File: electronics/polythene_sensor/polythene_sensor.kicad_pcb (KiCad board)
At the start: 2 copper layers, 8 parts, among them J1 Conn_02x16_Counter_Clockwise

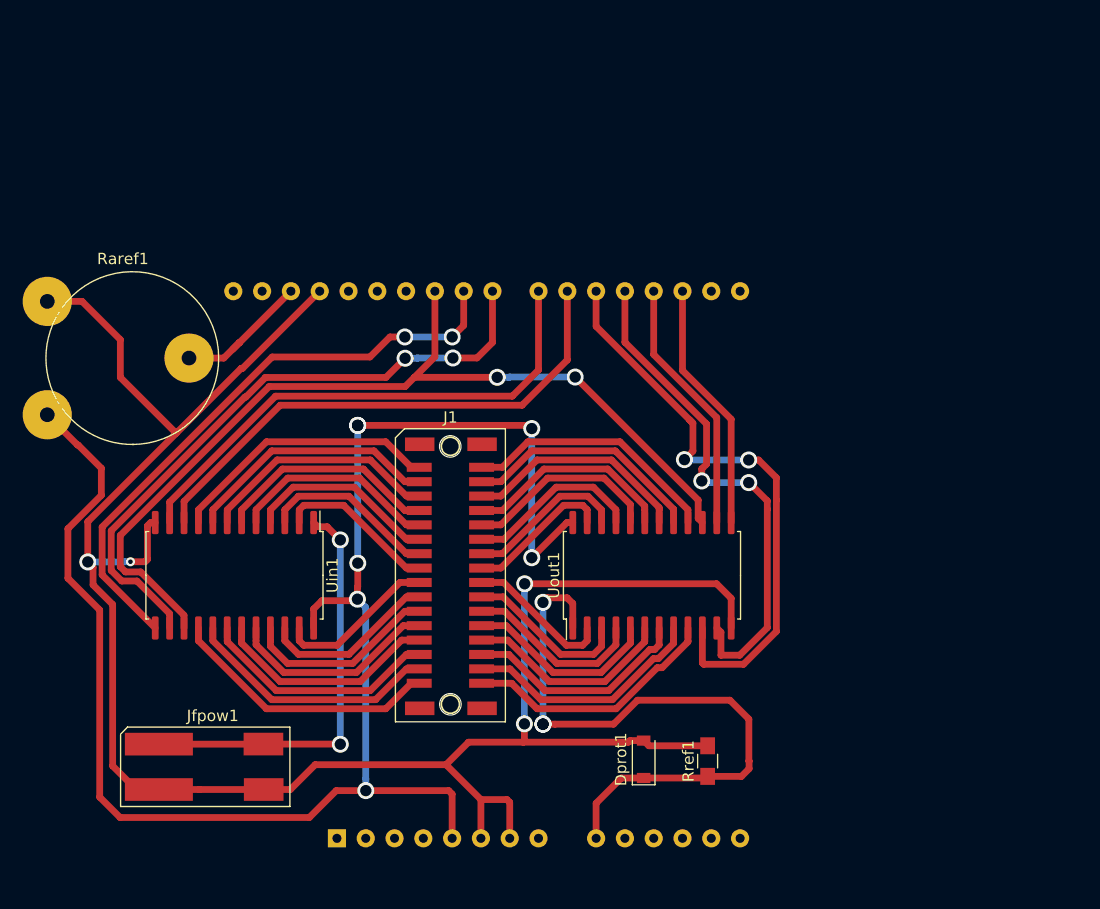
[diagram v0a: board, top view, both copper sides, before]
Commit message: Updated in the electronics
Signed-off-by: byteofsoren <r00tr4t@gmail.com>
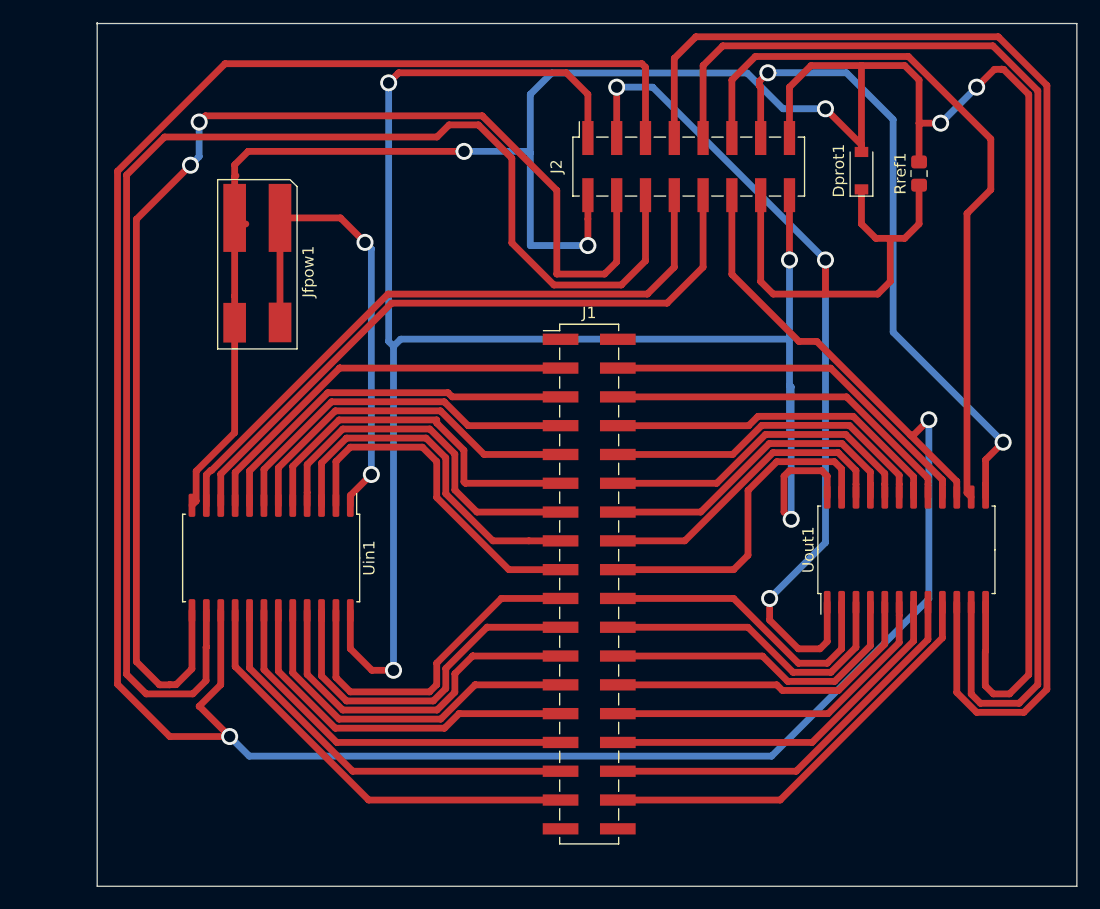
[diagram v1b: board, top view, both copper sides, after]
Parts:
- removed A1: Arduino_UNO_R3, Module:Arduino_UNO_R3
- removed Raref1: 10k, Potentiometer_THT:Potentiometer_Piher_PT-15-V02_Vertical
- added J2: Conn_02x08_Odd_Even, Connector_PinSocket_2.54mm:PinSocket_2x08_P2.54mm_Vertical_SMD, F.Cu at (177.8, 58.4)
- Dprot1: footprint Diodes_SMD:D_SOD-123 -> Diode_SMD:D_SOD-123
- J1: value Conn_02x16_Counter_Clockwise -> Conn_02x18_Odd_Even; footprint One27:One27_male_32pin -> Connector_PinHeader_2.54mm:PinHeader_2x18_P2.54mm_Vertical_SMD
- Rref1: footprint Resistors_SMD:R_0805_HandSoldering -> Resistor_SMD:R_0805_2012Metric_Pad1.15x1.40mm_HandSolder
- moved Dprot1 55.4 mm to (193.0, 58.8)
- moved Rref1 55.1 mm to (198.1, 59.1)
- moved Jfpow1 43.8 mm to (139.8, 67.7), turned to 180 degrees
- moved Uout1 22.6 mm to (197.0, 92.2)
- moved J1 12.3 mm to (169.0, 95.3), turned to 0 degrees
- moved Uin1 3.58 mm to (141.0, 93.0)
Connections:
- Uin1 pad 16: Net-(J1-Pad16) -> Net-(J1-Pad33)
- Uin1 pad 17: Net-(J1-Pad15) -> Net-(J1-Pad31)
- Uin1 pad 18: Net-(J1-Pad14) -> Net-(J1-Pad29)
- Uin1 pad 19: Net-(J1-Pad13) -> Net-(J1-Pad27)
- Uin1 pad 2: Net-(J1-Pad8) -> Net-(J1-Pad17)
- Uin1 pad 20: Net-(J1-Pad12) -> Net-(J1-Pad25)
- Uin1 pad 21: Net-(J1-Pad11) -> Net-(J1-Pad23)
- Uin1 pad 22: Net-(J1-Pad10) -> Net-(J1-Pad21)
- Uin1 pad 23: Net-(J1-Pad9) -> Net-(J1-Pad19)
- Uin1 pad 3: Net-(J1-Pad7) -> Net-(J1-Pad15)
- Uin1 pad 4: Net-(J1-Pad6) -> Net-(J1-Pad13)
- Uin1 pad 5: Net-(J1-Pad5) -> Net-(J1-Pad11)
- Uin1 pad 6: Net-(J1-Pad4) -> Net-(J1-Pad9)
- Uin1 pad 7: Net-(J1-Pad3) -> Net-(J1-Pad7)
- Uin1 pad 8: Net-(J1-Pad2) -> Net-(J1-Pad5)
- Uin1 pad 9: Net-(J1-Pad1) -> Net-(J1-Pad3)
- Uout1 pad 16: Net-(J1-Pad32) -> Net-(J1-Pad4)
- Uout1 pad 17: Net-(J1-Pad31) -> Net-(J1-Pad6)
- Uout1 pad 18: Net-(J1-Pad30) -> Net-(J1-Pad8)
- Uout1 pad 19: Net-(J1-Pad29) -> Net-(J1-Pad10)
- Uout1 pad 2: Net-(J1-Pad24) -> Net-(J1-Pad20)
- Uout1 pad 20: Net-(J1-Pad28) -> Net-(J1-Pad12)
- Uout1 pad 21: Net-(J1-Pad27) -> Net-(J1-Pad14)
- Uout1 pad 22: Net-(J1-Pad26) -> Net-(J1-Pad16)
- Uout1 pad 23: Net-(J1-Pad25) -> Net-(J1-Pad18)
- Uout1 pad 3: Net-(J1-Pad23) -> Net-(J1-Pad22)
- Uout1 pad 4: Net-(J1-Pad22) -> Net-(J1-Pad24)
- Uout1 pad 5: Net-(J1-Pad21) -> Net-(J1-Pad26)
- Uout1 pad 6: Net-(J1-Pad20) -> Net-(J1-Pad28)
- Uout1 pad 7: Net-(J1-Pad19) -> Net-(J1-Pad30)
- Uout1 pad 8: Net-(J1-Pad18) -> Net-(J1-Pad32)
- Uout1 pad 9: Net-(J1-Pad17) -> Net-(J1-Pad34)
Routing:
- net /EN: track 83.0 -> 248.8 mm
- net /S6: track 56.6 -> 122.9 mm, vias 2 -> 0
- net /S7: track 53.1 -> 114.9 mm
- net /S3: track 52.2 -> 113.2 mm, vias 2 -> 0
- net /S2: track 45.2 -> 105.6 mm, vias 2 -> 0
- net Net-(Dprot1-Pad1): track 57.9 -> 112.3 mm
- net /S1: track 22.7 -> 64.4 mm
- net Net-(J1-Pad33): track 0.00 -> 38.5 mm
- net GND: track 184.5 -> 222.5 mm, vias 4 -> 5
- net Net-(J1-Pad34): track 0.00 -> 37.7 mm
- net /S0: track 22.2 -> 56.8 mm, vias 0 -> 2
- net Net-(J1-Pad1): track 24.0 -> 0.00 mm
- net Net-(J1-Pad2): track 22.6 -> 0.00 mm
- net Net-(J1-Pad25): track 12.9 -> 32.1 mm
- net Net-(J1-Pad9): track 14.2 -> 31.9 mm
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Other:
- board outline added: 86.4 x 76.1 mm
